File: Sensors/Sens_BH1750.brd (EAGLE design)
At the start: 5.5 x 9.2 mm, 10 parts, among them IC1 BH1750FVI, X1 VCC, X3 SCL, X4 SDA

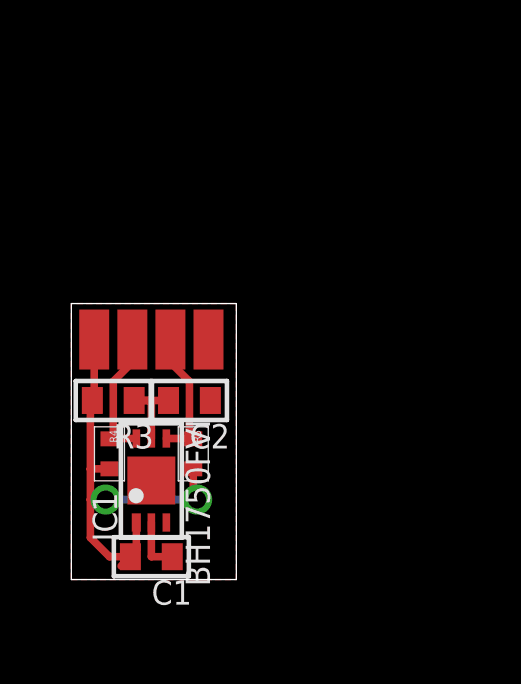
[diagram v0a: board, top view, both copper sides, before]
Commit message: Added S4M13
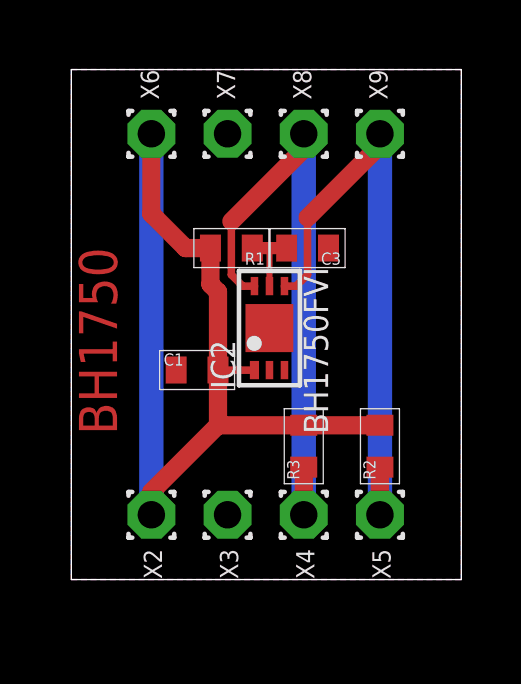
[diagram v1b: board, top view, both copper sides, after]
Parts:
- removed C2: 1u, RCL:0603
- removed IC1: BH1750FVI, Optic:WSOF6I
- removed R4, R5: 4k7, RCL:0402
- removed X1: VCC, Conn:S2.0/1.0
- added C3: 1u, RCL:0603
- added IC2: BH1750FVI, Optic:WSOF6I
- added R1: 1k, RCL:0603
- added R2: 10k, RCL:0603
- added X5, X9: SDA, Conn:T1.6/0.9
- added X6: 3v3, Conn:T1.6/0.9
- added X7: GND, Conn:T1.6/0.9
- added X8: SCL, Conn:T1.6/0.9
- R3: value 1k -> 10k
- X2: value (none) -> 3v3; device Conn:S2.0/1.0 -> Conn:T1.6/0.9
- X3: value SCL -> GND; device Conn:S2.0/1.0 -> Conn:T1.6/0.9
- X4: value SDA -> SCL; device Conn:S2.0/1.0 -> Conn:T1.6/0.9
- moved X4 7.34 mm to (7.75, 2.16), turned to 270 degrees
- moved X3 6.65 mm to (5.21, 2.16), turned to 270 degrees
- moved R3 6.53 mm to (7.75, 4.45), turned to 90 degrees
- moved C1 6.41 mm to (4.19, 6.99), turned to 0 degrees
- moved X2 6.14 mm to (2.67, 2.16), turned to 270 degrees
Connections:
- removed net N$2: C2.2, IC1.5, R3.1
- removed net N$3: C1.2, IC1.1, R3.2, R4.2, R5.2, X1.1
- new net +3V3: C1.2, IC2.1, R1.2, R2.2, R3.2, X2.1, X6.1
- new net N$1: C3.2, IC2.5, R1.1
- net GND: now also C3.1, IC2.2, IC2.3, X3.1, X7.1; no longer C2.1, IC1.2, IC1.3, X2.1
- net SCL: now also IC2.6, R3.1, X4.1, X8.1; no longer IC1.6, R4.1, X3.1
- net SDA: now also IC2.4, R2.1, X5.1, X9.1; no longer IC1.4, R5.1, X4.1
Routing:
- net +3V3: track 0.00 -> 34.4 mm
- net SCL: track 4.60 -> 20.9 mm
- net SDA: track 4.60 -> 20.9 mm
- net N$3: track 15.3 -> 0.00 mm, vias 2 -> 0
- net N$2: track 2.98 -> 0.00 mm
- net N$1: track 0.00 -> 2.41 mm
- net GND: track 1.78 -> 0.00 mm
- added copper zone on layer 16, net GND
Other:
- board size 5.5 x 9.2 mm -> 13 x 17 mm
- board text added: "BH1750"
